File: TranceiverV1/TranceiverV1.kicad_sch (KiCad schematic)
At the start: 6 parts, among them J1 Conn_01x03_Socket, J3 Conn_01x02_Socket, J4 Conn_01x03_Pin, J5 Conn_02x04_Odd_Even, M1 Motor_Servo, U3 102010388

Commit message: designed first iteration of pcb
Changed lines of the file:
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@@
+	(wire
+		(pts
+			(xy 139.7 43.18) (xy 146.05 43.18)
+		)
+		(stroke
+			(width 0)
+			(type default)
+		)
+	)
 	(wire
 		(pts
@@
 	(wire
 		(pts
-			(xy 146.05 43.18) (xy 139.7 43.18)
-		)
-		(stroke
-			(width 0)
-			(type default)
-		)
-	)
-	(wire
-		(pts
 			(xy 120.65 43.18) (xy 127 43.18)
 		)
@@
 	(label "CE"
 		(at 96.52 67.31 0)
-		(effects
-			(font
-				(size 1.27 1.27)
-			)
-			(justify left bottom)
-		)
-	)
-	(label "IRQ"
-		(at 146.05 43.18 0)
 		(effects
 			(font
@@
 		)
 	)
+	(label "IRQ"
+		(at 146.05 43.18 0)
+		(effects
+			(font
+				(size 1.27 1.27)
+			)
+			(justify left bottom)
+		)
+	)

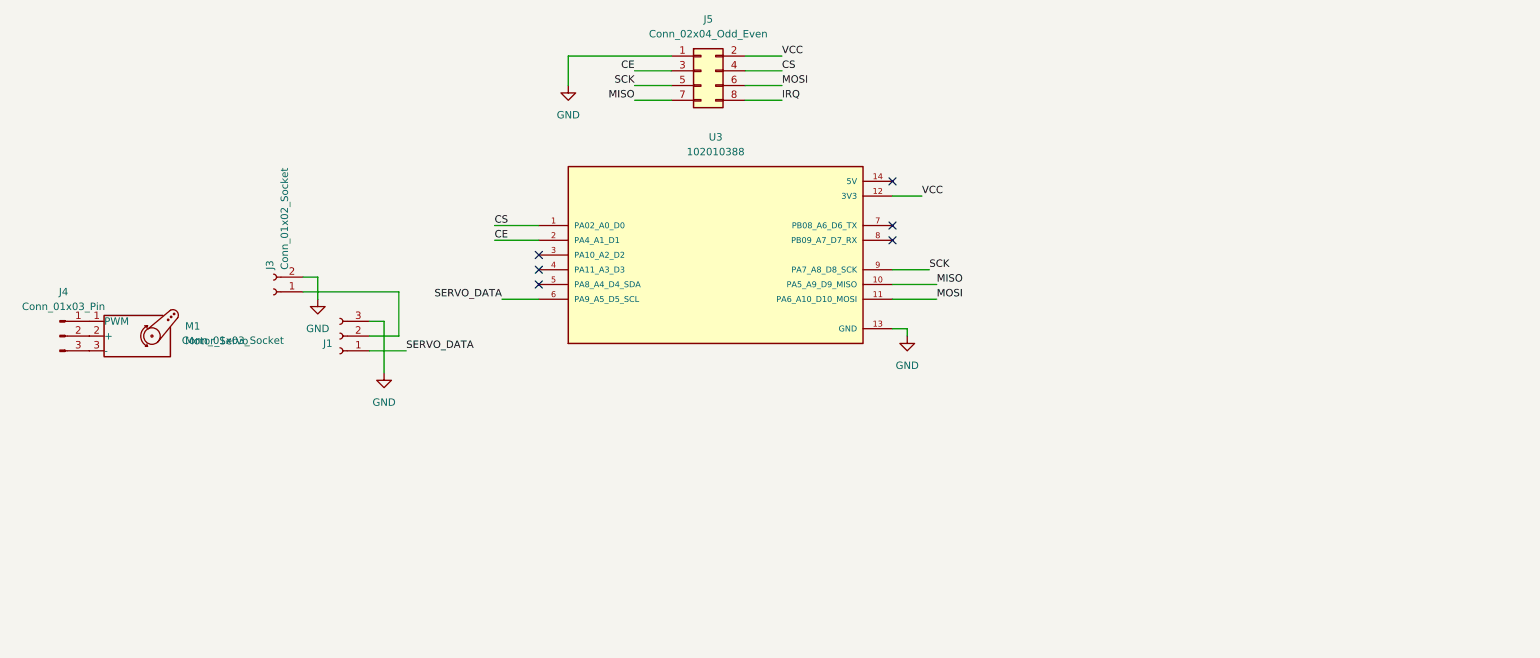
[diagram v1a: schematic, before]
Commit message: updated schematic for pcb iteration
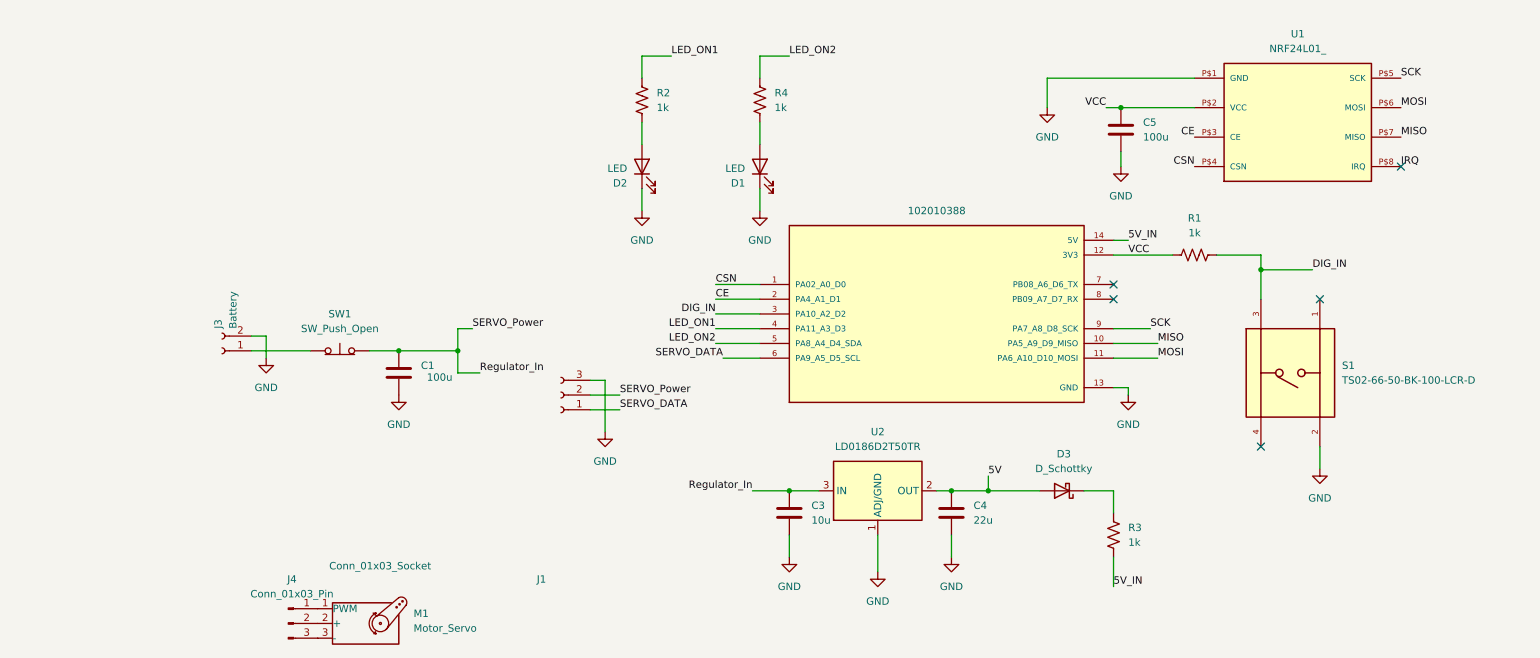
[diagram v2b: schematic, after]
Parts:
- removed J5: Conn_02x04_Odd_Even, Connector_PinHeader_2.54mm:PinHeader_2x04_P2.54mm_Vertical, symbol Connector_Generic:Conn_02x04_Odd_Even
- added C1, C5: 100u, symbol Device:C
- added C3: 10u, symbol Device:C
- added C4: 22u, symbol Device:C
- added D1, D2: LED, LED_THT:LED_D5.0mm, symbol Device:LED
- added D3: D_Schottky, symbol Device:D_Schottky
- added R1, R3: 1k, symbol Device:R_US
- added R2, R4: 1k, Resistor_THT:R_Axial_DIN0204_L3.6mm_D1.6mm_P2.54mm_Vertical, symbol Device:R_US
- added S1: TS02-66-50-BK-100-LCR-D, TS02_66_50_BK_100_LCR_D_Folder:SW_TS02-66-50-BK-100-LCR-D, symbol TS02-66-50-BK-100-LCR-D:TS02-66-50-BK-100-LCR-D
- added SW1: SW_Push_Open, Button_Switch_THT:SW_PUSH_1P1T_6x3.5mm_H5.0_APEM_MJTP1250, symbol Switch:SW_Push_Open
- added U1: NRF24L01_, RF_Module:nRF24L01_Breakout, symbol NRF24L01_:NRF24L01_
- added U2: LD0186D2T50TR, Package_TO_SOT_SMD:TO-263-2, symbol Regulator_Linear:LD0186D2T50TR
- J3: value Conn_01x02_Socket -> Battery
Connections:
- net CE: now also U1.P$3 (CE)
- net GND: now also C1.2, C3.2, C4.2, C5.2, D1.1 (K), D2.1 (K), S1.2, U1.P$1 (GND), U2.1 (ADJ/GND)
- net IRQ: now also U1.P$8 (IRQ)
- net MISO: now also U1.P$7 (MISO)
- net MOSI: now also U1.P$6 (MOSI)
- net SCK: now also U1.P$5 (SCK)
- net VCC: now also C5.1, R1.1, U1.P$2 (VCC)
- net 5V_IN: now reaches U3.14 (5V)
- net 5V_IN: now also R3.2
- net DIG_IN: now reaches U3.3 (PA10_A2_D2)
- net DIG_IN: now also R1.2, S1.3
- net LED_ON1: now reaches U3.4 (PA11_A3_D3)
- net LED_ON1: now also R2.1
- net LED_ON2: now reaches U3.5 (PA8_A4_D4_SDA)
- net LED_ON2: now also R4.1
- net at J3.1 (Pin_1): now also SW1.1 (A); no longer J1.2 (Pin_2)
- net CS renamed CSN
- net CSN: now also U1.P$4 (CSN)
- new net: D2.2 (A), R2.2
- new net: D3.1 (K), R3.1
- new net: D1.2 (A), R4.2
- new net 5V: C4.1, D3.2 (A), U2.2 (OUT)
- new net Regulator_In: C1.1, C3.1, J1.2 (Pin_2), SW1.2 (B), U2.3 (IN)
- no-connect marks 6 -> 5
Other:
- moved on the sheet: J1, J3, J4, M1
